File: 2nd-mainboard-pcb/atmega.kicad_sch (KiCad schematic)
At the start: 16 parts, among them U10 ATmega328PB-A, Y1 ECS-160-18-4X-CKM

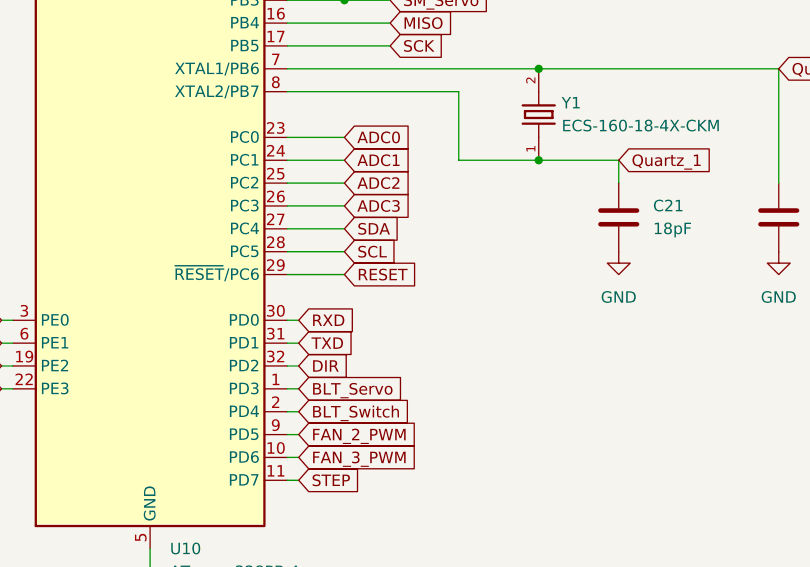
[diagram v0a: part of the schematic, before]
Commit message: last few changes
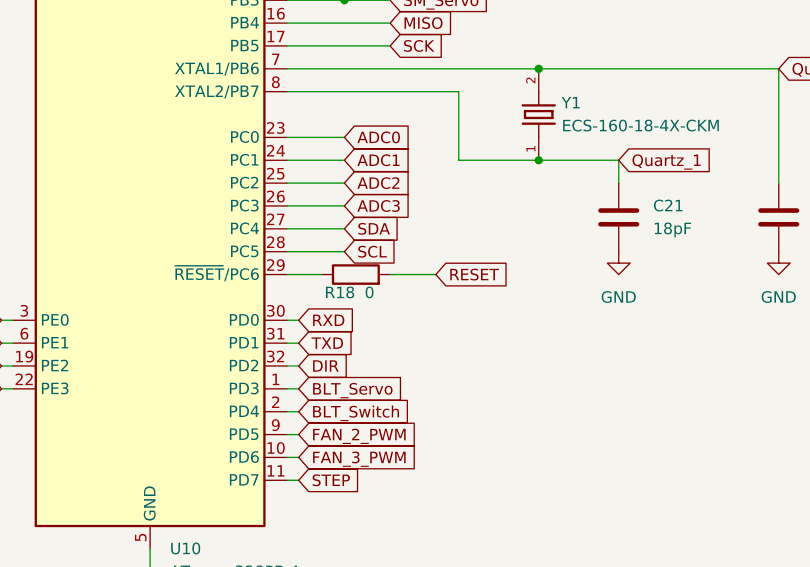
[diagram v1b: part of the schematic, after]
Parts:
- added R18: 0, Resistor_SMD:R_0603_1608Metric_Pad0.98x0.95mm_HandSolder, symbol Device:R
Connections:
- net RESET: now also R18.2; no longer U10.29 (~{RESET}/PC6)
- new net: R18.1, U10.29 (~{RESET}/PC6)
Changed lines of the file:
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@@
 	(wire
 		(pts
+			(xy 104.14 101.6) (xy 109.22 101.6)
+		)
+		(stroke
+			(width 0)
+			(type default)
+		)
+	)
+	(wire
+		(pts
 			(xy 198.12 74.93) (xy 198.12 73.66)
 		)
@@
 	(wire
 		(pts
-			(xy 92.71 101.6) (xy 99.06 101.6)
+			(xy 92.71 101.6) (xy 96.52 101.6)
 		)
 		(stroke
@@
 	(global_label "RESET"
 		(shape input)
-		(at 99.06 101.6 0)
+		(at 109.22 101.6 0)
 		(fields_autoplaced yes)
 		(effects
@@
 		)
 		(property "Intersheetrefs" "${INTERSHEET_REFS}"
-			(at 107.7903 101.6 0)
+			(at 117.9503 101.6 0)
 			(effects
 				(font
@@
 					(unit 1)
 				)
+			)
+		)
+	)
+	(symbol
+		(lib_id "Device:R")
+		(at 100.33 101.6 90)
+		(unit 1)
+		(exclude_from_sim no)
+		(in_bom yes)
+		(on_board yes)
+		(dnp no)
+		(property "Reference" "R18"
+			(at 98.552 103.632 90)
+			(effects
+				(font
+					(size 1.27 1.27)
+				)
+			)
+		)
+		(property "Value" "0"
+			(at 101.854 103.632 90)
+			(effects
+				(font
+					(size 1.27 1.27)
+				)
+			)
+		)
+		(property "Footprint" "Resistor_SMD:R_0603_1608Metric_Pad0.98x0.95mm_HandSolder"
+			(at 100.33 103.378 90)
+			(effects
+				(font
+					(size 1.27 1.27)
+				)
+				(hide yes)
+			)
+		)
+		(property "Datasheet" "~"
+			(at 100.33 101.6 0)
+			(effects
+				(font
+					(size 1.27 1.27)
+				)
+				(hide yes)
+			)
+		)
+		(property "Description" "Resistor"
+			(at 100.33 101.6 0)
+			(effects
+				(font
+					(size 1.27 1.27)
+				)
+				(hide yes)
+			)
+		)
+		(pin "1"
+		)
+		(pin "2"
+		)
+		(instances
+			(project ""
+				(path "/6926a609-8b92-4b3a-88c8-3d023174b977/2814f85c-0b7e-4ab3-b3e5-bcf29424baab"
+					(reference "R18")
+					(unit 1)
+				)
